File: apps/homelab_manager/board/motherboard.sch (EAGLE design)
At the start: 39 parts, among them X1 22-23-2021

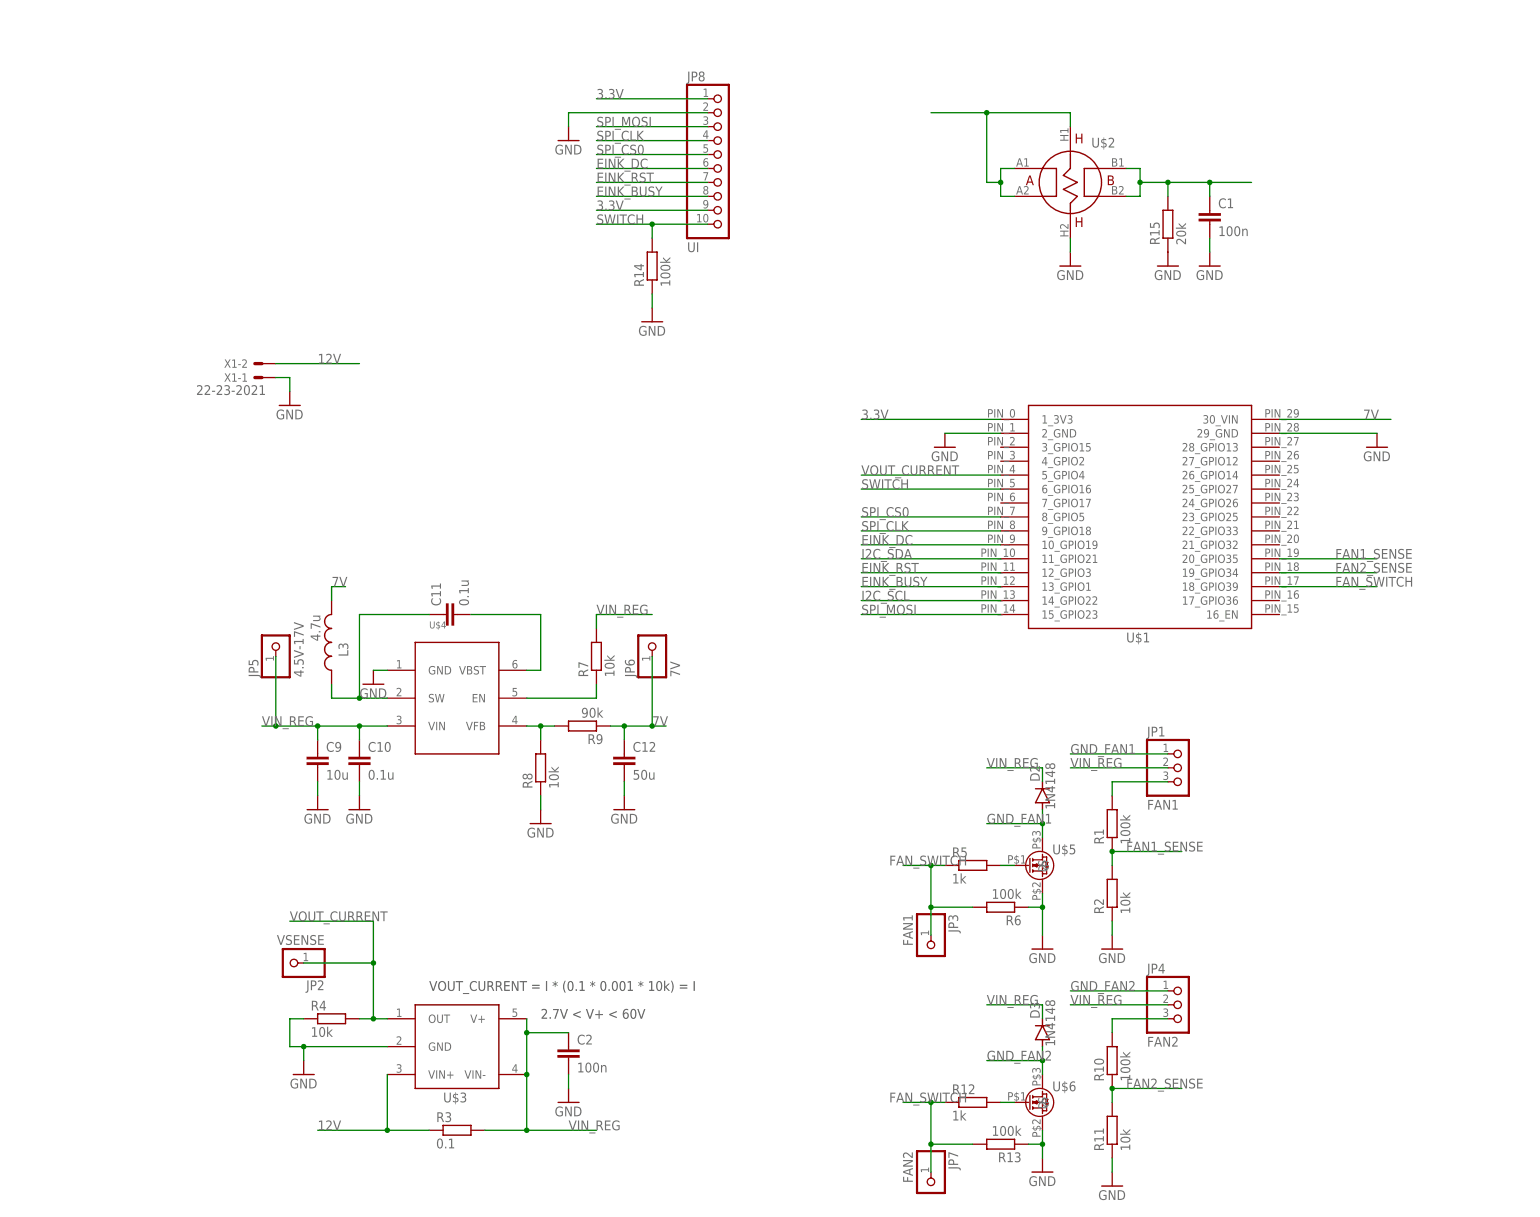
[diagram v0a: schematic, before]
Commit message: Adding components
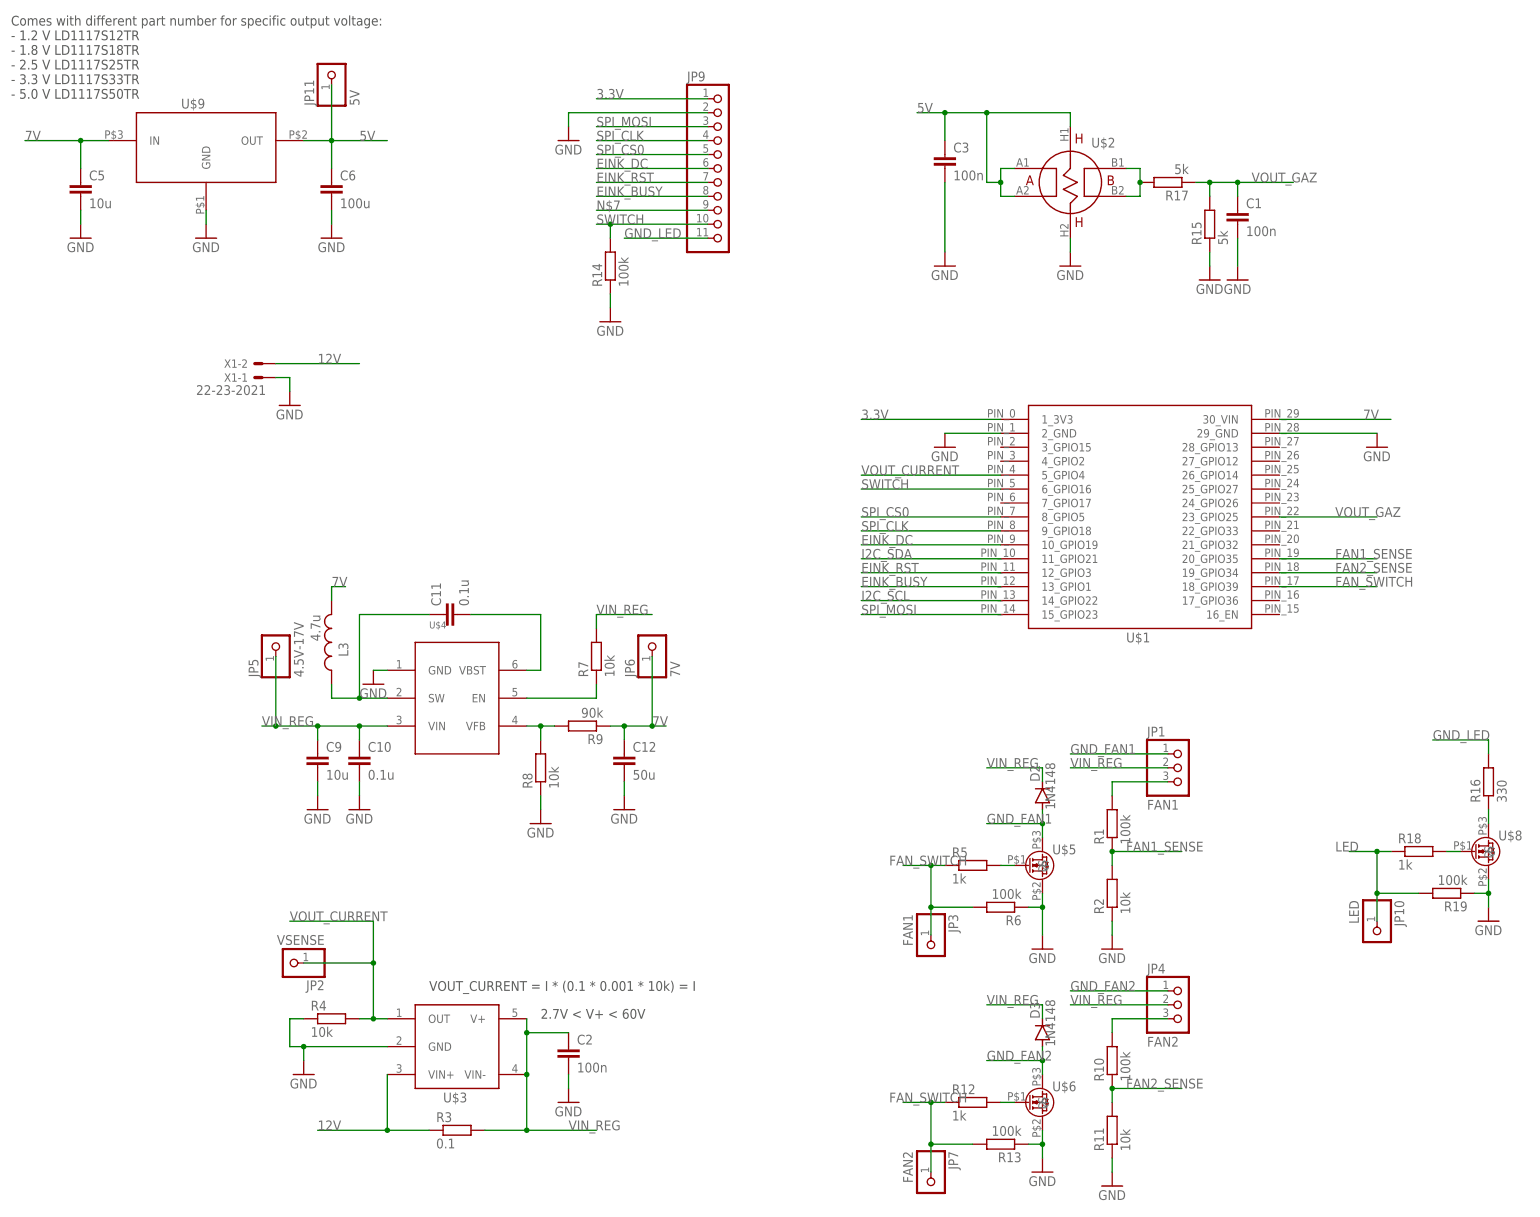
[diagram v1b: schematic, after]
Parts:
- removed JP8: UI, pinhead:PINHD-1X10
- added C3: 100n, rcl:C-EUC0805
- added C5: 10u, rcl:C-EUC0805
- added C6: 100u, rcl:C-EUC0805
- added JP10: LED, pinhead:PINHD-1X1
- added JP11: 5V, pinhead:PINHD-1X1
- added JP9: (no value), pinhead:PINHD-1X11
- added R16: 330, rcl:R-EU_R0805
- added R17: 5k, rcl:R-EU_R0805
- added R18: 1k, rcl:R-EU_R0805
- added R19: 100k, rcl:R-EU_R0805
- added U$8: MGSF1N03L, bzd:MGSF1N03L
- added U$9: LD1117, bzd:LD1117
- R15: value 20k -> 5k
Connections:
- removed net N$6: C1.1, R15.2, U$2.B1, U$2.B2
- new net 5V: C3.1, C6.1, JP11.1, U$2.A1, U$2.A2, U$2.H1, U$9.OUT
- new net GND_LED: JP9.11, R16.2
- new net LED: JP10.1, R18.1, R19.2
- new net N$14: R16.1, U$8.D
- new net N$7: JP9.9
- new net N$8: R18.2, U$8.G
- new net VOUT_GAZ: C1.1, R15.2, R17.1, U$1.23_GPIO25
- net 3.3V: now also JP9.1; no longer JP8.1, JP8.9
- net 7V: now also C5.1, U$9.IN
- net EINK_BUSY: now also JP9.8; no longer JP8.8
- net EINK_DC: now also JP9.6; no longer JP8.6
- net EINK_RST: now also JP9.7; no longer JP8.7
- net GND: now also C3.2, C5.2, C6.2, JP9.2, R19.1, U$8.S, U$9.GND; no longer JP8.2
- net N$5: now also R17.2, U$2.B1, U$2.B2; no longer U$2.A1, U$2.A2, U$2.H1
- net SPI_CLK: now also JP9.4; no longer JP8.4
- net SPI_CS0: now also JP9.5; no longer JP8.5
- net SPI_MOSI: now also JP9.3; no longer JP8.3
- net SWITCH: now also JP9.10; no longer JP8.10
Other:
- note added: "Comes with different part number for specific output voltage: - 1.2 V LD1117S12TR - 1.8 V LD1117S18TR - 2.5 V LD1117S25TR - 3.3 V LD1117S33TR - 5.0 V LD1117S50TR"
- moved on the sheet: C1, R14, R15
